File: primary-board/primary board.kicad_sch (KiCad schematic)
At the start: 29 parts, among them J1 USB_C, J10 Motor Connector Right, J5 I2C Breakout, J9 Motor Connector Left, SW1 SW_SPST, SW2 SW_SPST, U1 ESP32-S3-1, U5 DRV8411ARTER

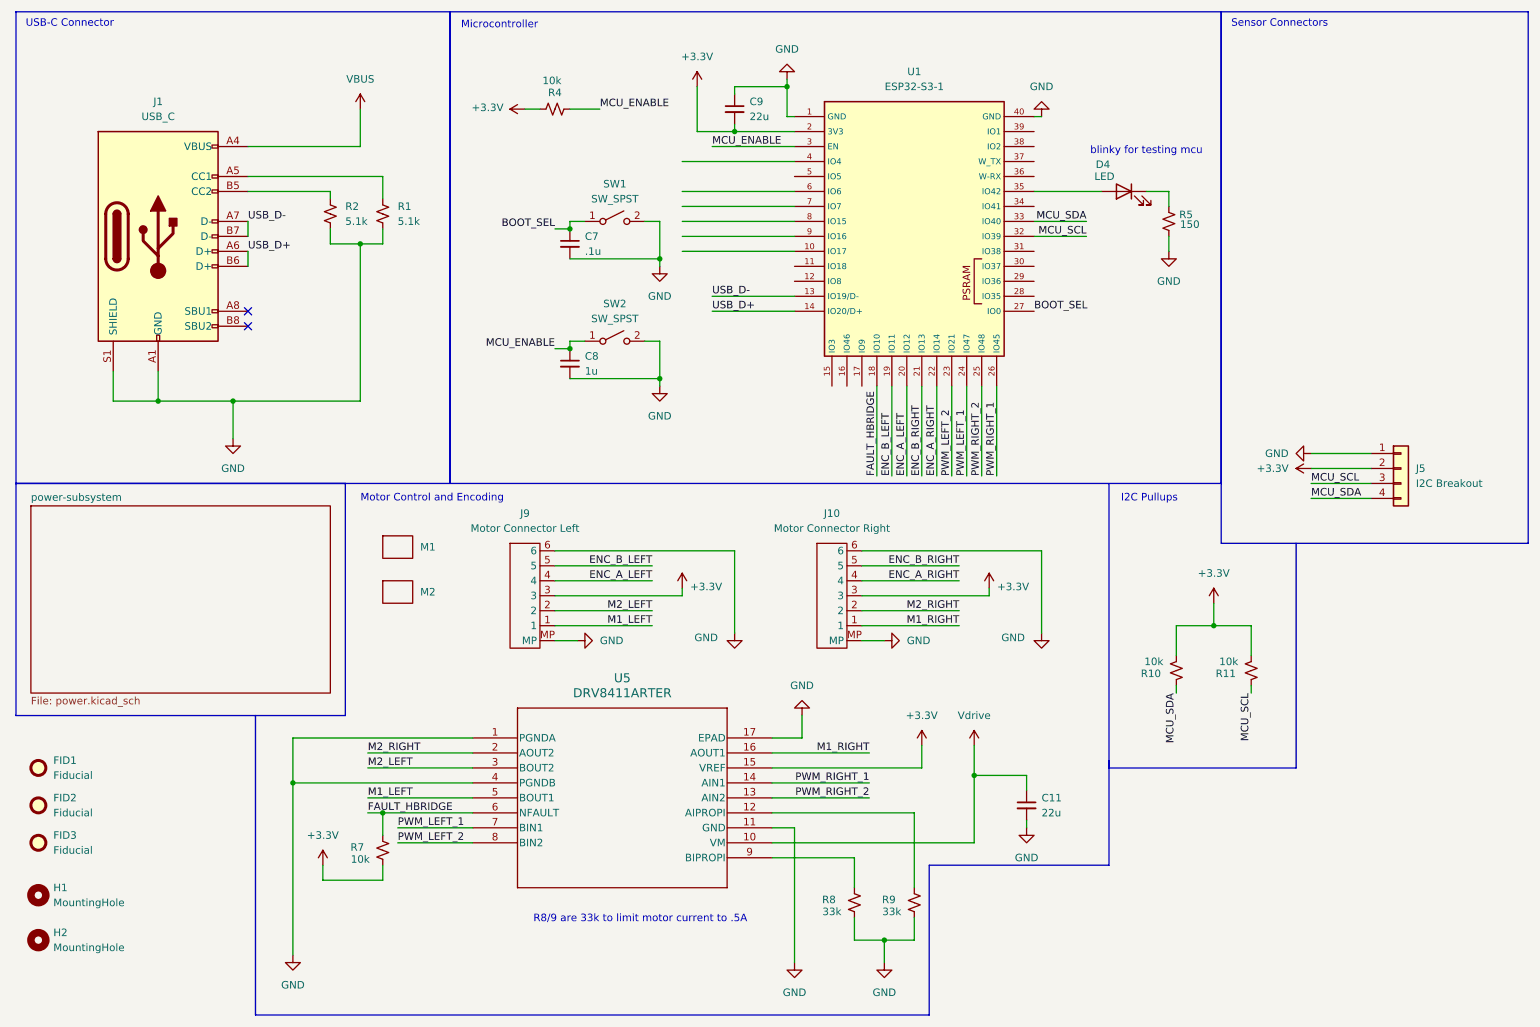
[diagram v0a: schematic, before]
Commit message: analog work
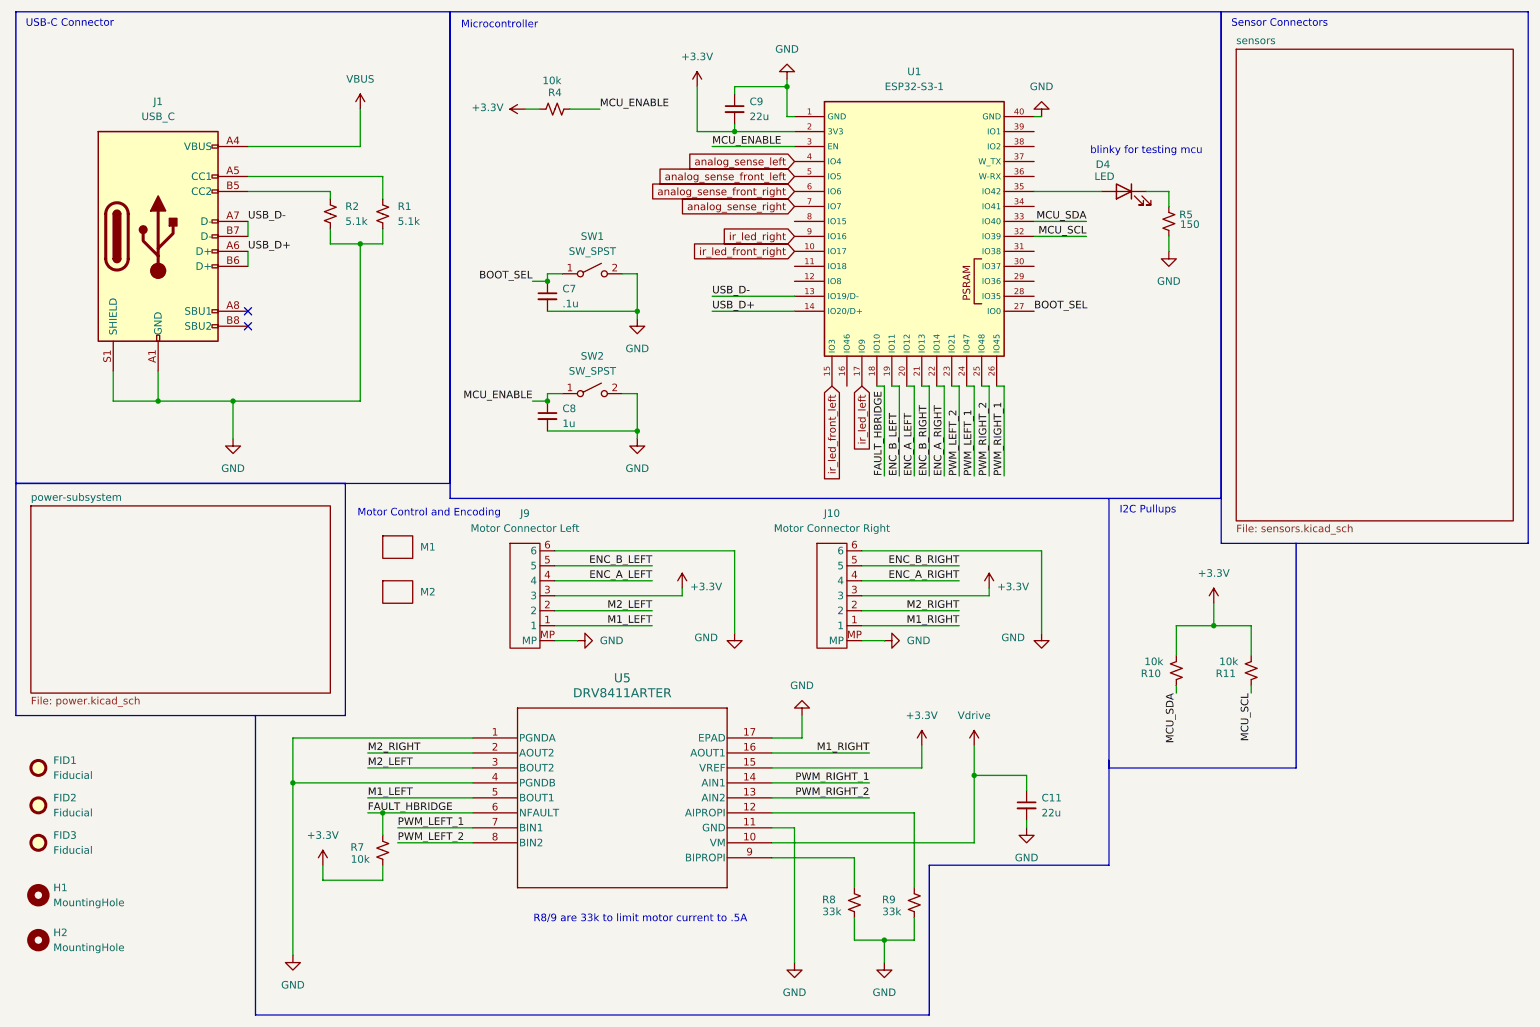
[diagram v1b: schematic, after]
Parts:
- removed J5: I2C Breakout, Connector_PinSocket_2.54mm:PinSocket_1x04_P2.54mm_Vertical, symbol Connector_Generic:Conn_01x04
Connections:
- net ir_led_front_right: now reaches U1.10 (IO17)
- net ir_led_front_left: now reaches U1.15 (IO3)
- net ir_led_left: now reaches U1.17 (IO9)
- net analog_sense_left: now reaches U1.4 (IO4)
- net analog_sense_front_left: now reaches U1.5 (IO5)
- net analog_sense_front_right: now reaches U1.6 (IO6)
- net analog_sense_right: now reaches U1.7 (IO7)
- net ir_led_right: now reaches U1.9 (IO16)
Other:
- added sheet sensors (sensors.kicad_sch)
- moved on the sheet: C7, C8, SW1, SW2
